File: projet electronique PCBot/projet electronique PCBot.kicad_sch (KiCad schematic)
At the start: 0 parts

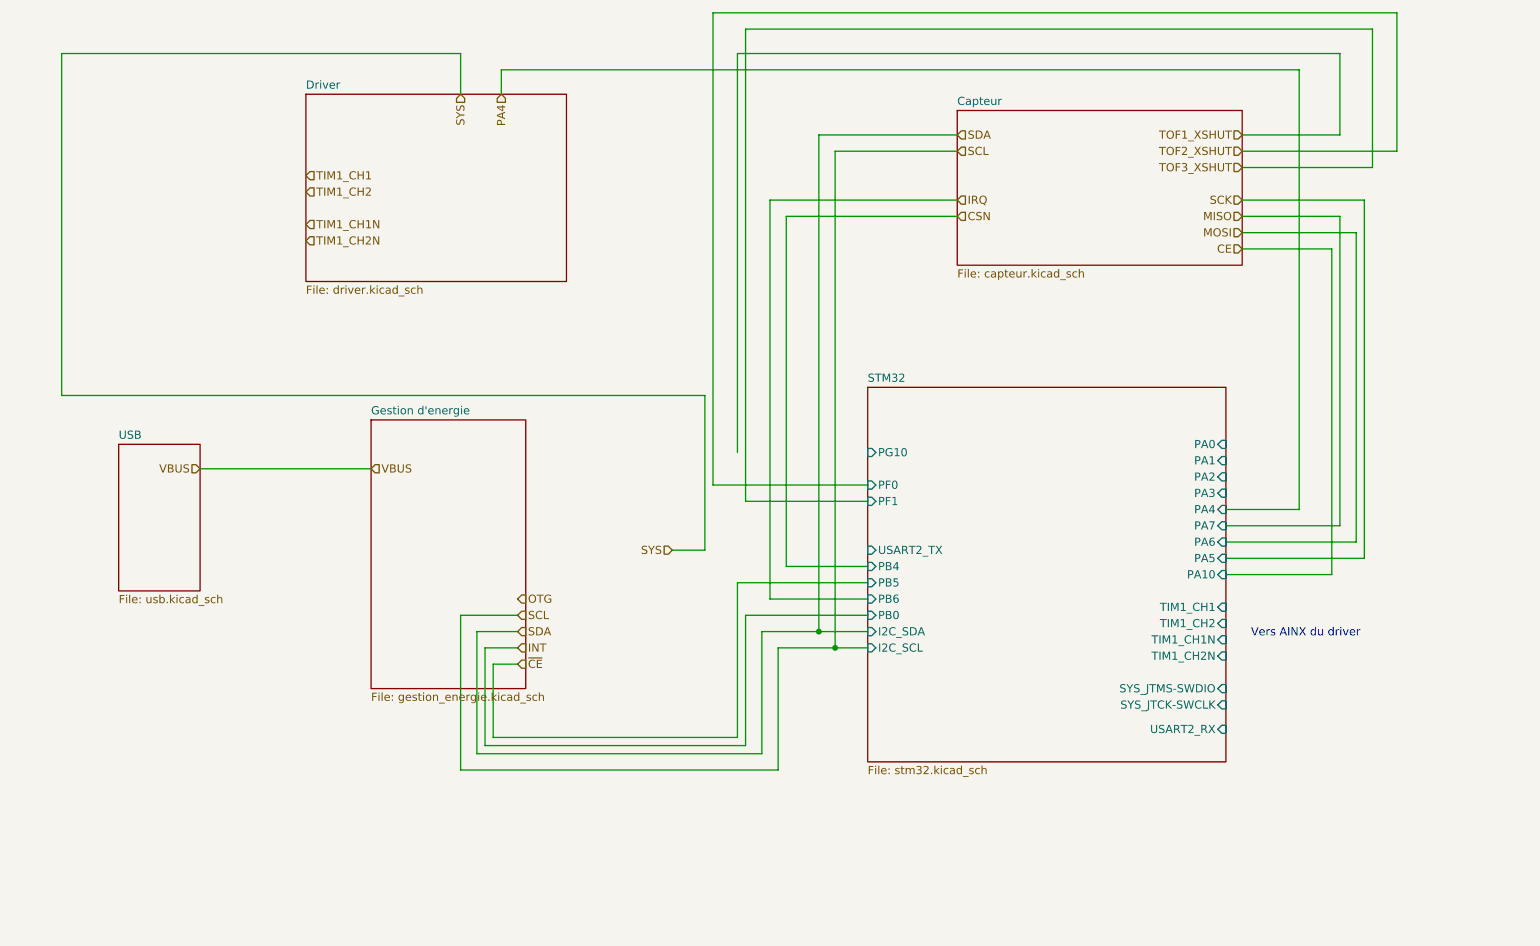
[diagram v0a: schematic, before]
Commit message: modif après revu prof
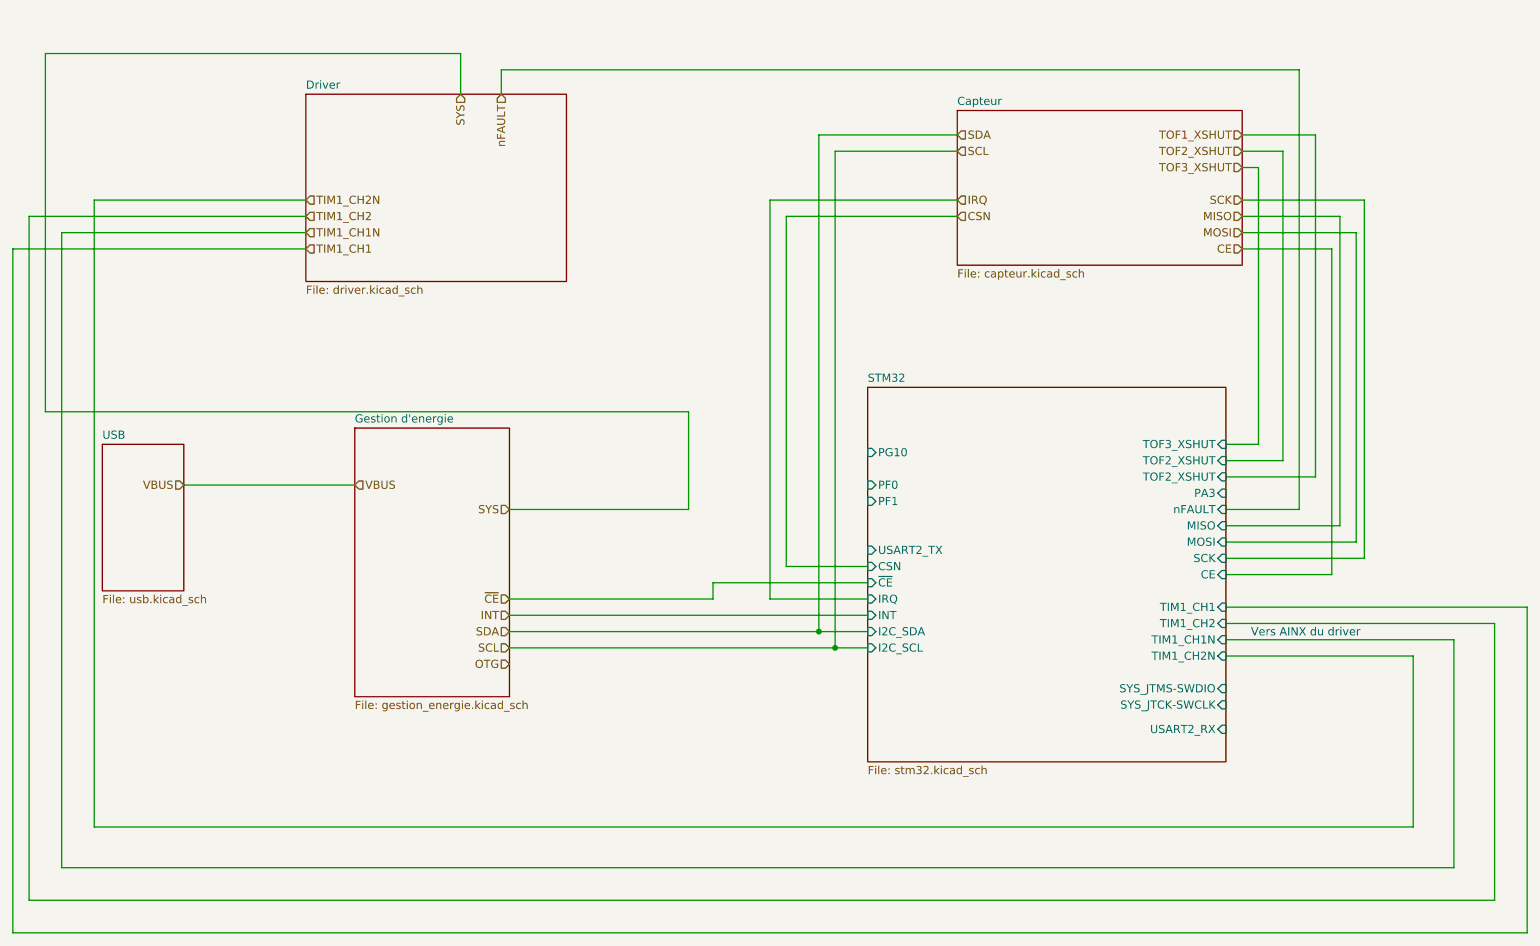
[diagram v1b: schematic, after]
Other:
- sheet STM32 ports: added CE, CSN, INT, IRQ, MISO, MOSI, SCK, TOF2_XSHUT, TOF3_XSHUT, nFAULT, ~{CE}; removed PA0, PA1, PA10, PA2, PA4, PA5, PA6, PA7, PB0, PB4, PB5, PB6
